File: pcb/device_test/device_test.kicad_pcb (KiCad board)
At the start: 4 copper layers, 55 x 55 mm, 0 parts

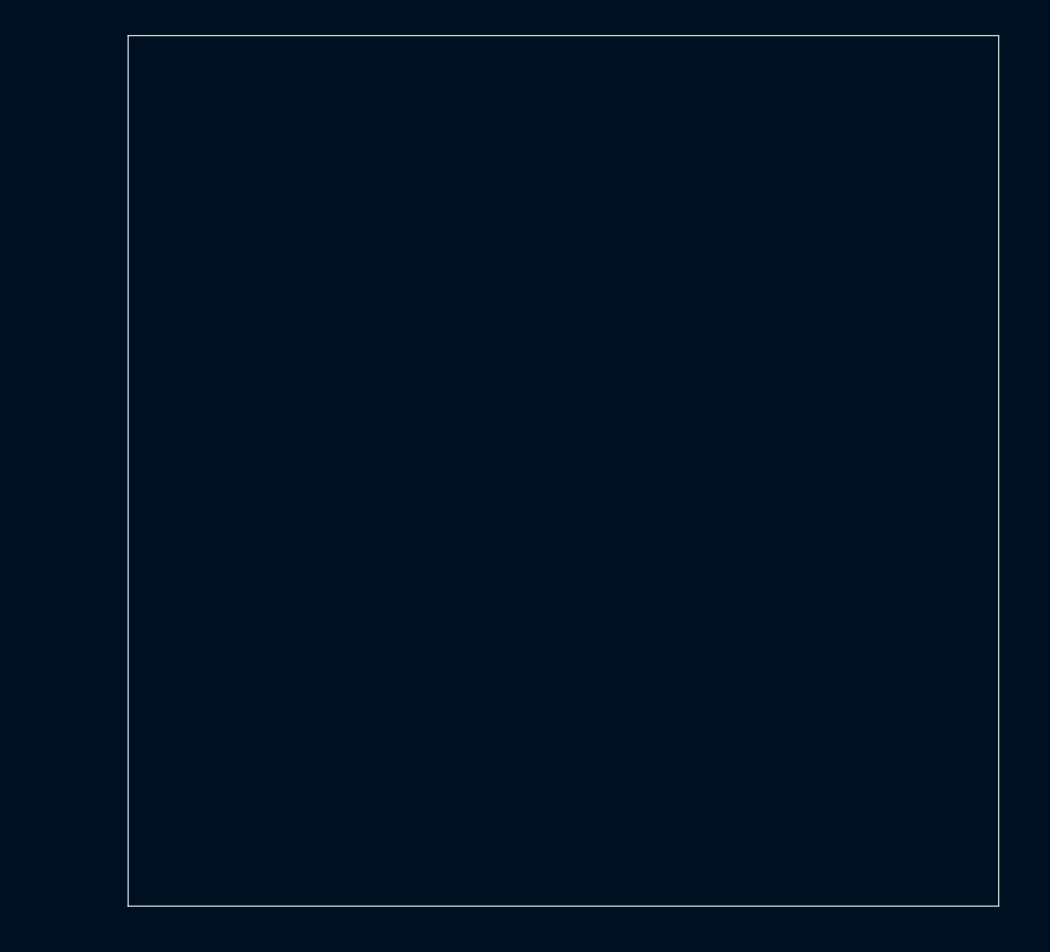
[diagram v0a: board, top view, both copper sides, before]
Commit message: pcb update
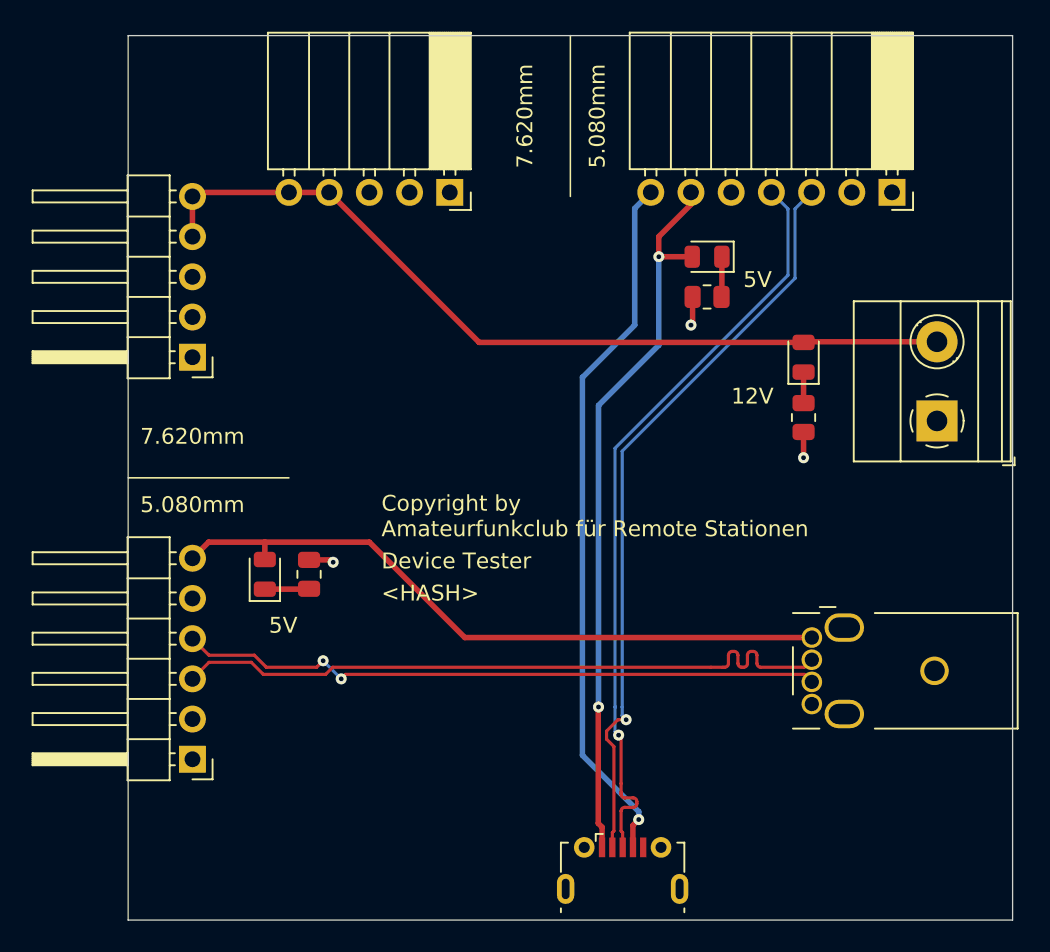
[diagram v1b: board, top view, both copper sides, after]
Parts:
- added D101: LED, LED_SMD:LED_0805_2012Metric, F.Cu at (158.4, 83.6)
- added D102: LED, LED_SMD:LED_0805_2012Metric, F.Cu at (152.3, 77.2)
- added D103: LED, LED_SMD:LED_0805_2012Metric, F.Cu at (124.4, 97.3)
- added J101: Screw_Terminal_01x02, TerminalBlock_Phoenix:TerminalBlock_Phoenix_MKDS-1,5-2_1x02_P5.00mm_Horizontal, F.Cu at (166.9, 87.6)
- added J102: Conn_01x05, Connector_PinSocket_2.54mm:PinSocket_1x05_P2.54mm_Horizontal, F.Cu at (136.1, 73.2)
- added J103: Conn_01x05, Connector_PinHeader_2.54mm:PinHeader_1x05_P2.54mm_Horizontal, F.Cu at (119.8, 83.6)
- added J104: USB_OTG, USB:MicroUSB-920-E52A2021S10100, F.Cu at (147.0, 116.0)
- added J105: USB_A, USB:USB_A_C456020, F.Cu at (160.0, 103.4)
- added J106: Conn_01x07, Connector_PinSocket_2.54mm:PinSocket_1x07_P2.54mm_Horizontal, F.Cu at (164.0, 73.1)
- added J107: Conn_01x06, Connector_PinHeader_2.54mm:PinHeader_1x06_P2.54mm_Horizontal, F.Cu at (119.8, 109.0)
- added R101: 1k8, Resistor_SMD:R_0805_2012Metric, F.Cu at (158.4, 87.4)
- added R102: 360, Resistor_SMD:R_0805_2012Metric, F.Cu at (152.3, 79.8)
- added R103: 360, Resistor_SMD:R_0805_2012Metric, F.Cu at (127.2, 97.3)
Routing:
- net +12V: track 0.00 -> 53.6 mm
- net /USB1+: track 0.00 -> 48.1 mm, vias 0 -> 1
- net /USB1-: track 0.00 -> 47.5 mm, vias 0 -> 1
- net +5V_A: track 0.00 -> 46.0 mm, vias 0 -> 2
- net /USB_OTG_ID: track 0.00 -> 44.8 mm, vias 0 -> 1
- net /USB2-: track 0.00 -> 43.4 mm
- net +5V_B: track 0.00 -> 43.1 mm
- net /USB2+: track 0.00 -> 40.8 mm, vias 0 -> 2
- net GND: track 0.00 -> 5.03 mm, vias 0 -> 3
- net Net-(D103-K): track 0.00 -> 2.80 mm
- net Net-(D102-K): track 0.00 -> 2.55 mm
- net Net-(D101-K): track 0.00 -> 1.96 mm
- added copper zone on In1.Cu, net GND
- added copper zone on In2.Cu, net GND
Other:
- board size 55 x 55 mm -> 55.9 x 55.9 mm
- board text added: "12V"
- board text added: "5.080mm"
- board text added: "5V"
- board text added: "7.620mm"
- board text added: "<HASH>"
- board text added: "Copyright by Amateurfunkclub für Remote Stationen"
- board text added: "Device Tester"
